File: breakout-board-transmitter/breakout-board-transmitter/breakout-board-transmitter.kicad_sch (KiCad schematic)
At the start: 19 parts, among them U1 CC1100-RTR1, Y1 Crystal

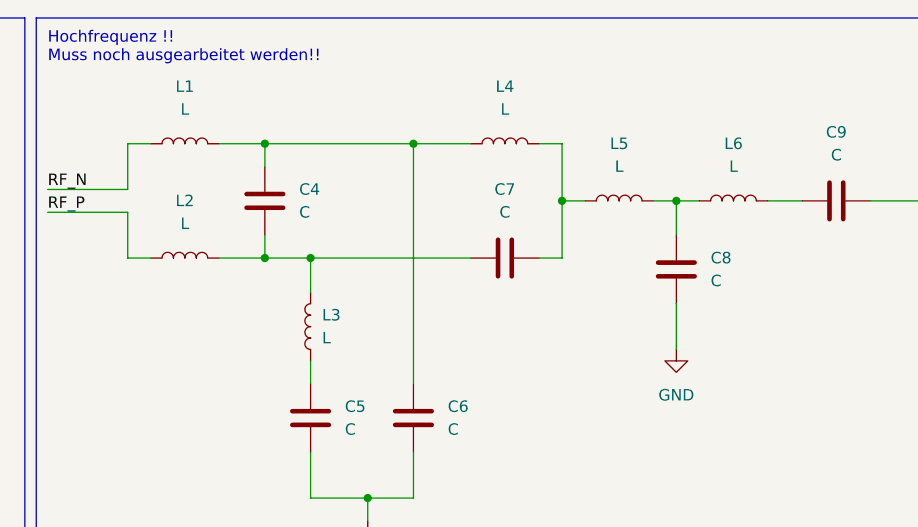
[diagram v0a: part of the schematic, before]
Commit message: Revert "..."
This reverts commit 6093de15b6a411821706cd1d809fe7ad2ca1dc62.
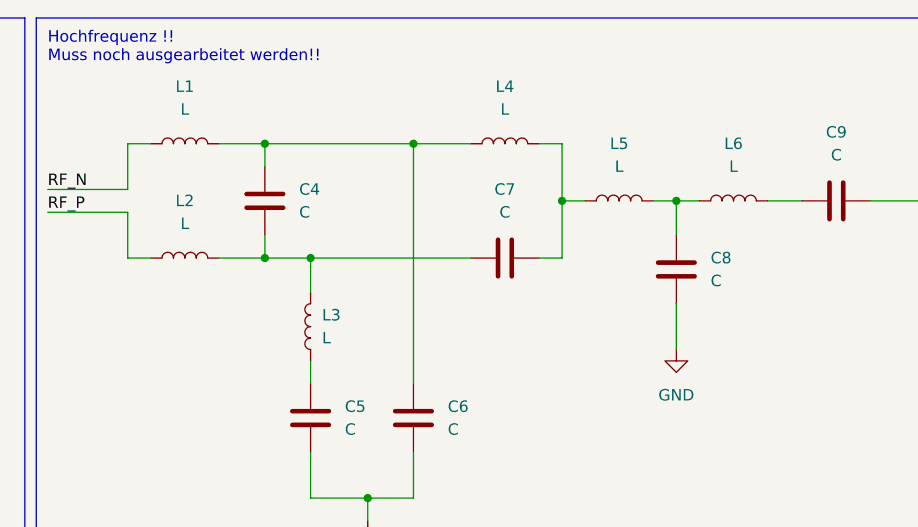
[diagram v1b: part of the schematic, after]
